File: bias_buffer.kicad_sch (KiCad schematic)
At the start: 5 parts, among them U22 PE4312C-Z

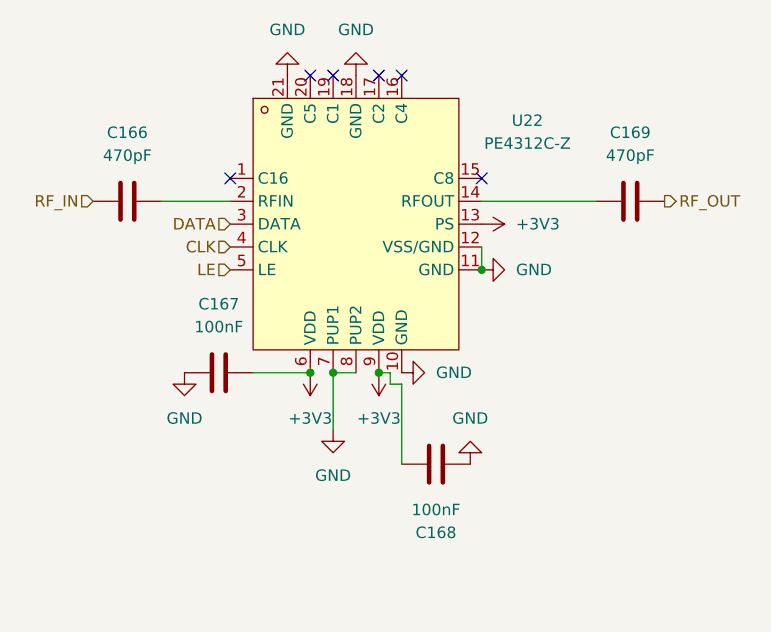
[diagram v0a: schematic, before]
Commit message: almost done with schematic
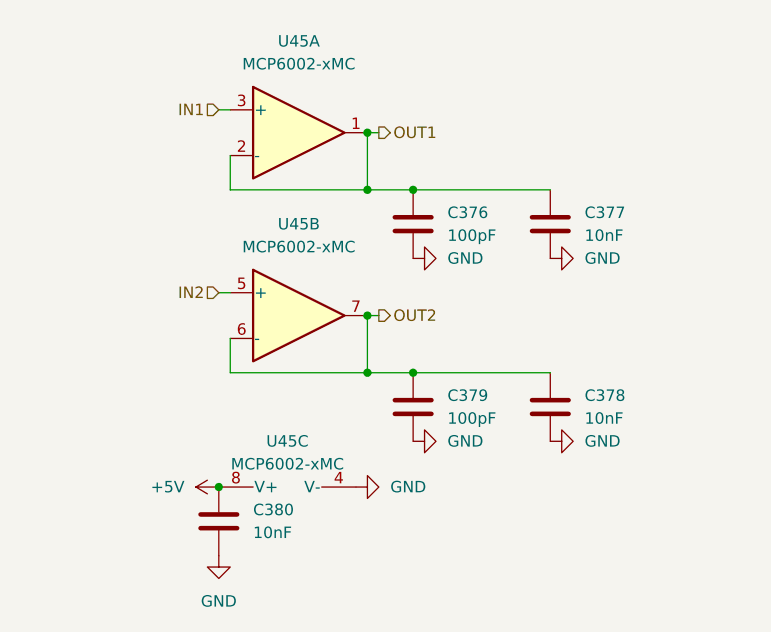
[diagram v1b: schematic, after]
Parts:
- removed C166, C169: 470pF, Capacitor_SMD:C_0402_1005Metric_Pad0.74x0.62mm_HandSolder, symbol Device:C
- removed C167, C168: 100nF, Capacitor_SMD:C_0402_1005Metric_Pad0.74x0.62mm_HandSolder, symbol Device:C
- removed U22: PE4312C-Z, easyeda2kicad:QFN-20_L4.0-W4.0-P0.50-BL-EP2.2, symbol easyeda2kicad:PE4312C-Z
- added C376, C379: 100pF, Capacitor_SMD:C_0402_1005Metric, symbol Device:C
- added C377, C378, C380: 10nF, Capacitor_SMD:C_0402_1005Metric, symbol Device:C
- added U45: MCP6002-xMC, Package_DFN_QFN:DFN-8-1EP_3x2mm_P0.5mm_EP1.75x1.45mm, symbol Amplifier_Operational:MCP6002-xMC
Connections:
- net GND: now also C376.2, C377.2, C378.2, C379.2, C380.2, U45.4 (V-), U45.9 (V-)
- new net +5V: C380.1, U45.8 (V+)
- new net IN1: U45.3 (+)
- new net IN2: U45.5 (+)
- new net OUT1: C376.1, C377.1, U45.1, U45.2 (-)
- new net OUT2: C378.1, C379.1, U45.6 (-), U45.7
- no-connect marks 6 -> 0
